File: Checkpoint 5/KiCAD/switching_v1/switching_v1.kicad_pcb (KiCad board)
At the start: 2 copper layers, 24 parts, among them J1 Conn_01x02, J2 Conn_01x02, U1 LM7809_TO220, U2 LM393, U4 TL072

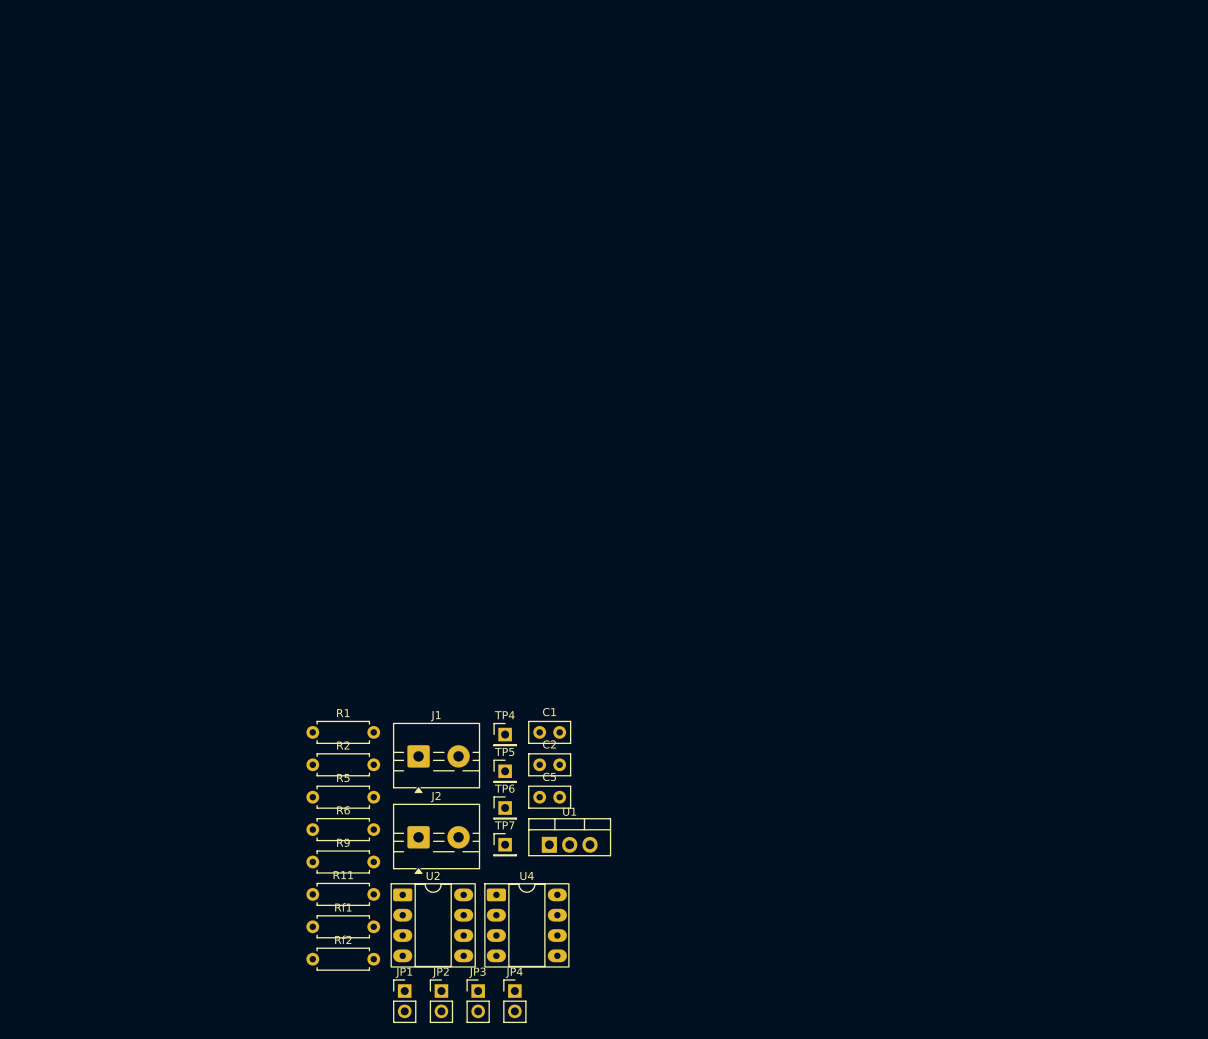
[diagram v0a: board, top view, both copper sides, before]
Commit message: avances PCB
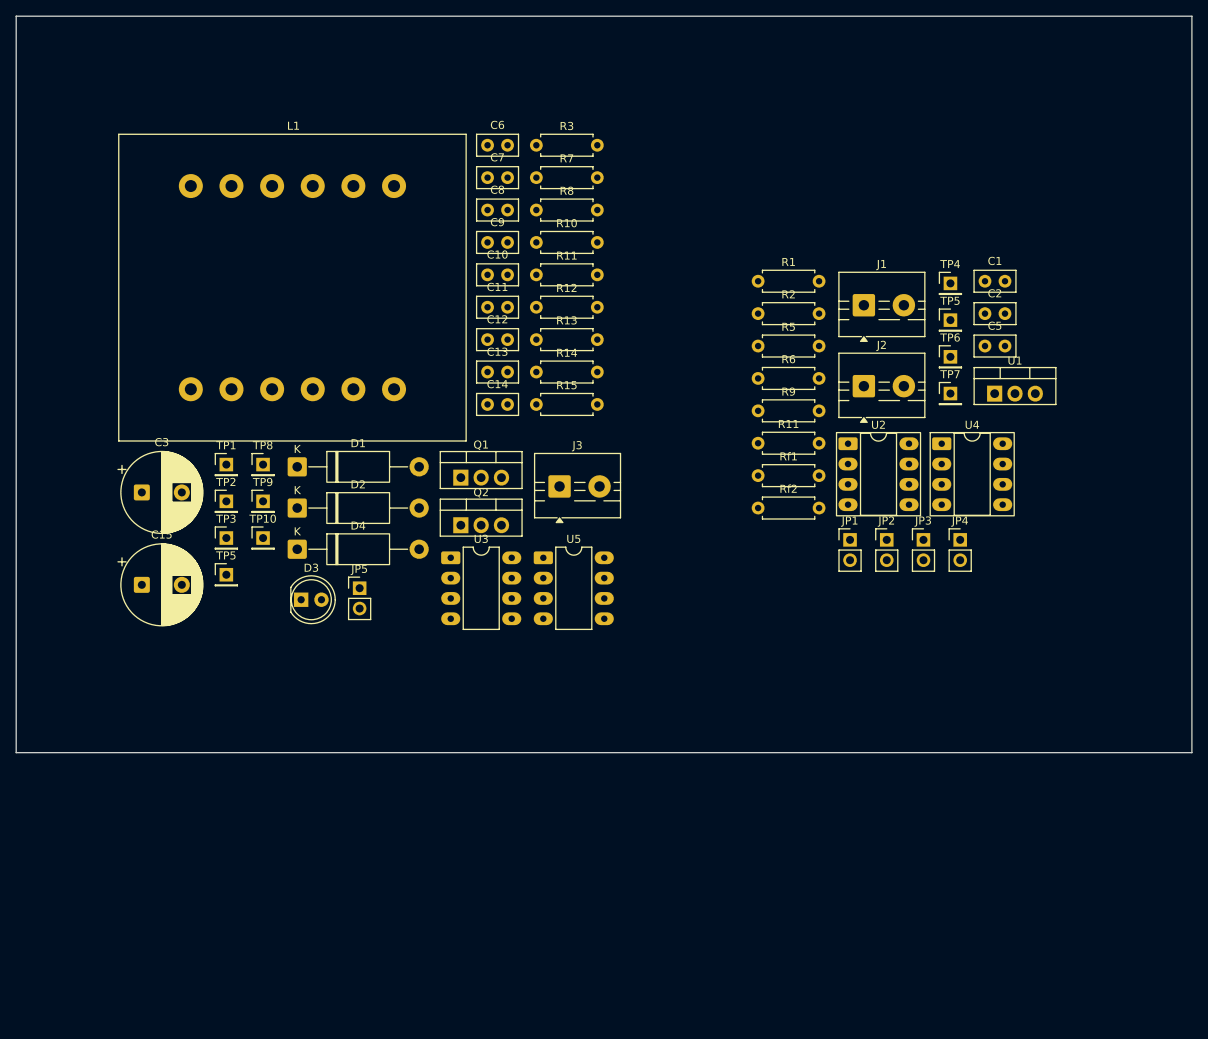
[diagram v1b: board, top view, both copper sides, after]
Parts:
- added C10: 0.1u, Capacitor_THT:C_Disc_D5.0mm_W2.5mm_P2.50mm, F.Cu at (149.9, 81.3)
- added C11: C, Capacitor_THT:C_Disc_D5.0mm_W2.5mm_P2.50mm, F.Cu at (149.9, 85.4)
- added C12: C, Capacitor_THT:C_Disc_D5.0mm_W2.5mm_P2.50mm, F.Cu at (149.9, 89.4)
- added C13: C, Capacitor_THT:C_Disc_D5.0mm_W2.5mm_P2.50mm, F.Cu at (149.9, 93.5)
- added C14: 0.1u, Capacitor_THT:C_Disc_D5.0mm_W2.5mm_P2.50mm, F.Cu at (149.9, 97.5)
- added C15: C_Polarized, Capacitor_THT:CP_Radial_D10.0mm_P5.00mm, F.Cu at (106.7, 120.1)
- added C3: C_Polarized, Capacitor_THT:CP_Radial_D10.0mm_P5.00mm, F.Cu at (106.7, 108.5)
- added C6: C, Capacitor_THT:C_Disc_D5.0mm_W2.5mm_P2.50mm, F.Cu at (149.9, 65.1)
- added C7: 0.1u, Capacitor_THT:C_Disc_D5.0mm_W2.5mm_P2.50mm, F.Cu at (149.9, 69.2)
- added C8: 0.1u, Capacitor_THT:C_Disc_D5.0mm_W2.5mm_P2.50mm, F.Cu at (149.9, 73.2)
- added C9: 1u, Capacitor_THT:C_Disc_D5.0mm_W2.5mm_P2.50mm, F.Cu at (149.9, 77.3)
- added D1: D_Schottky, Diode_THT:D_DO-15_P15.24mm_Horizontal, F.Cu at (126.1, 105.3)
- added D2: D_Schottky, Diode_THT:D_DO-15_P15.24mm_Horizontal, F.Cu at (126.1, 110.5)
- added D3: LED, LED_THT:LED_D5.0mm_IRGrey, F.Cu at (126.6, 121.9)
- added D4: D_Schottky, Diode_THT:D_DO-15_P15.24mm_Horizontal, F.Cu at (126.1, 115.6)
- added J3: Conn_01x02, TerminalBlock:TerminalBlock_MaiXu_MX126-5.0-02P_1x02_P5.00mm, F.Cu at (158.9, 107.8)
- added JP5: SD_IN, Connector_PinHeader_2.54mm:PinHeader_1x02_P2.54mm_Vertical, F.Cu at (133.9, 120.5)
- added L1: L, Transformer_THT:Transformer_37x44, F.Cu at (117.9, 70.2)
- added Q1: IRF740, Package_TO_SOT_THT:TO-220-3_Vertical, F.Cu at (146.6, 106.7)
- added Q2: IRF740, Package_TO_SOT_THT:TO-220-3_Vertical, F.Cu at (146.6, 112.6)
- added R10: 1, Resistor_THT:R_Axial_DIN0207_L6.3mm_D2.5mm_P7.62mm_Horizontal, F.Cu at (156.0, 77.3)
- added R11: 56k, Resistor_THT:R_Axial_DIN0207_L6.3mm_D2.5mm_P7.62mm_Horizontal, F.Cu at (156.0, 81.3)
- added R12: R, Resistor_THT:R_Axial_DIN0207_L6.3mm_D2.5mm_P7.62mm_Horizontal, F.Cu at (156.0, 85.4)
- added R13: R, Resistor_THT:R_Axial_DIN0207_L6.3mm_D2.5mm_P7.62mm_Horizontal, F.Cu at (156.0, 89.4)
- added R14: R, Resistor_THT:R_Axial_DIN0207_L6.3mm_D2.5mm_P7.62mm_Horizontal, F.Cu at (156.0, 93.5)
- added R15: 5k1, Resistor_THT:R_Axial_DIN0207_L6.3mm_D2.5mm_P7.62mm_Horizontal, F.Cu at (156.0, 97.5)
- added R3: R, Resistor_THT:R_Axial_DIN0207_L6.3mm_D2.5mm_P7.62mm_Horizontal, F.Cu at (156.0, 65.1)
- added R7: 1, Resistor_THT:R_Axial_DIN0207_L6.3mm_D2.5mm_P7.62mm_Horizontal, F.Cu at (156.0, 69.2)
- added R8: 1, Resistor_THT:R_Axial_DIN0207_L6.3mm_D2.5mm_P7.62mm_Horizontal, F.Cu at (156.0, 73.2)
- added TP1: TestPoint, Connector_PinHeader_2.54mm:PinHeader_1x01_P2.54mm_Vertical, F.Cu at (117.3, 105.0)
- added TP10: TestPoint, Connector_PinHeader_2.54mm:PinHeader_1x01_P2.54mm_Vertical, F.Cu at (121.9, 114.2)
- added TP2: TestPoint, Connector_PinHeader_2.54mm:PinHeader_1x01_P2.54mm_Vertical, F.Cu at (117.3, 109.6)
- added TP3: TestPoint, Connector_PinHeader_2.54mm:PinHeader_1x01_P2.54mm_Vertical, F.Cu at (117.3, 114.2)
- added TP5: TP-Switching, Connector_PinHeader_2.54mm:PinHeader_1x01_P2.54mm_Vertical, F.Cu at (117.3, 118.8)
- added TP8: TestPoint, Connector_PinHeader_2.54mm:PinHeader_1x01_P2.54mm_Vertical, F.Cu at (121.9, 105.0)
- added TP9: TestPoint, Connector_PinHeader_2.54mm:PinHeader_1x01_P2.54mm_Vertical, F.Cu at (121.9, 109.6)
- added U3: IR2104, Package_DIP:DIP-8_W7.62mm_LongPads, F.Cu at (145.3, 116.7)
- added U5: TL071, Package_DIP:DIP-8_W7.62mm_LongPads, F.Cu at (156.9, 116.7)
- C5: value 33p -> 56p
- R5: value 150k -> 220k
- moved J1 79.2 mm to (197.0, 85.1)
- moved R1 79.2 mm to (183.7, 82.1)
- moved R11 79.2 mm to (183.7, 102.4)
- moved R6 79.2 mm to (183.7, 94.3)
- moved C1 79.2 mm to (212.1, 82.1)
- moved R5 79.2 mm to (183.7, 90.2)
- moved R9 79.2 mm to (183.7, 98.3)
- moved Rf2 79.2 mm to (183.7, 110.5)
- moved U2 79.2 mm to (195.0, 102.4)
- moved U4 79.2 mm to (206.7, 102.4)
- moved J2 79.2 mm to (197.0, 95.2)
- moved R2 79.2 mm to (183.7, 86.2)
- moved Rf1 79.2 mm to (183.7, 106.4)
- moved C2 79.2 mm to (212.1, 86.2)
- moved C5 79.2 mm to (212.1, 90.2)
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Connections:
- U2 pad 4: (no net) -> GND
- U2 pad 8: (no net) -> +9V
- U4 pad 4: (no net) -> GND
- U4 pad 5: /Vref_opamp -> /Vref
- U4 pad 8: (no net) -> +9V
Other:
- board outline added: 147 x 92.1 mm
